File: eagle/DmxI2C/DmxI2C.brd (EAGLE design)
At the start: 55 x 69.5 mm, 30 parts, among them IC2 MAX485, IC3 MEGA48/88/168-AU, Q1 20MHz

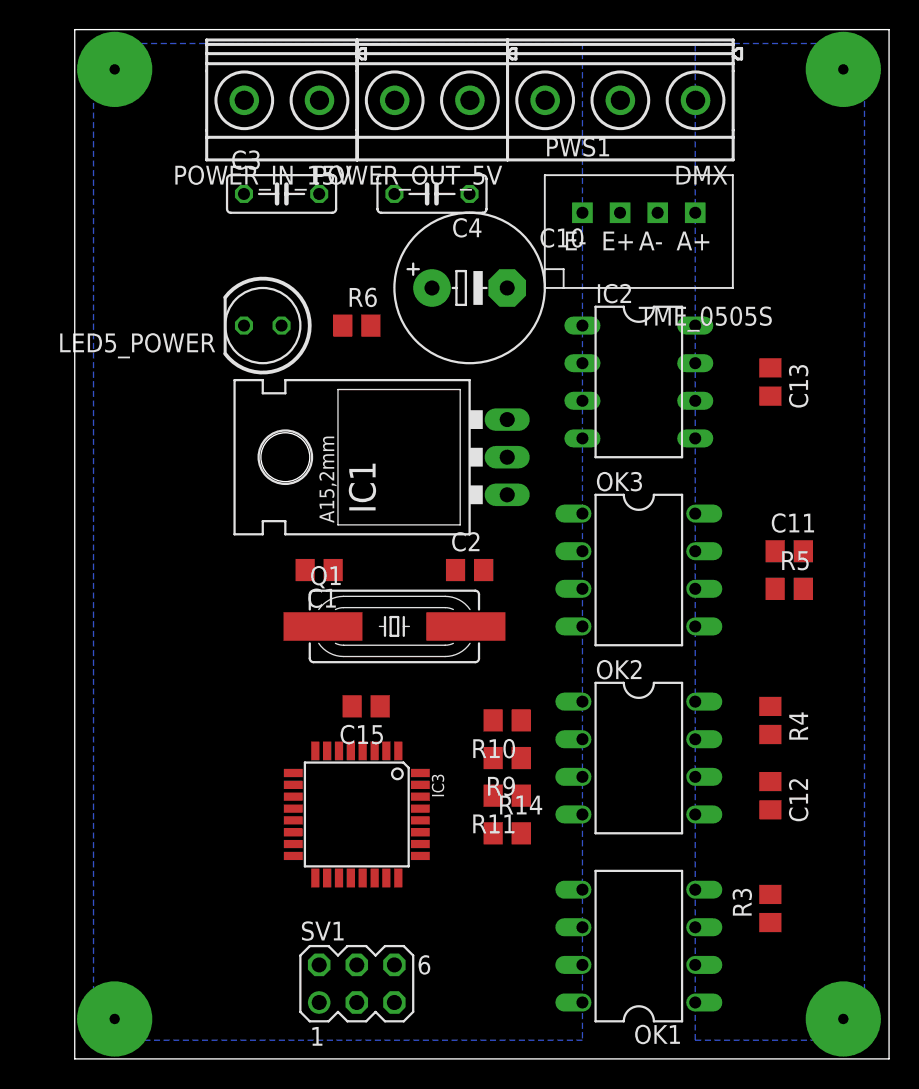
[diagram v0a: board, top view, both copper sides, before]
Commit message: .
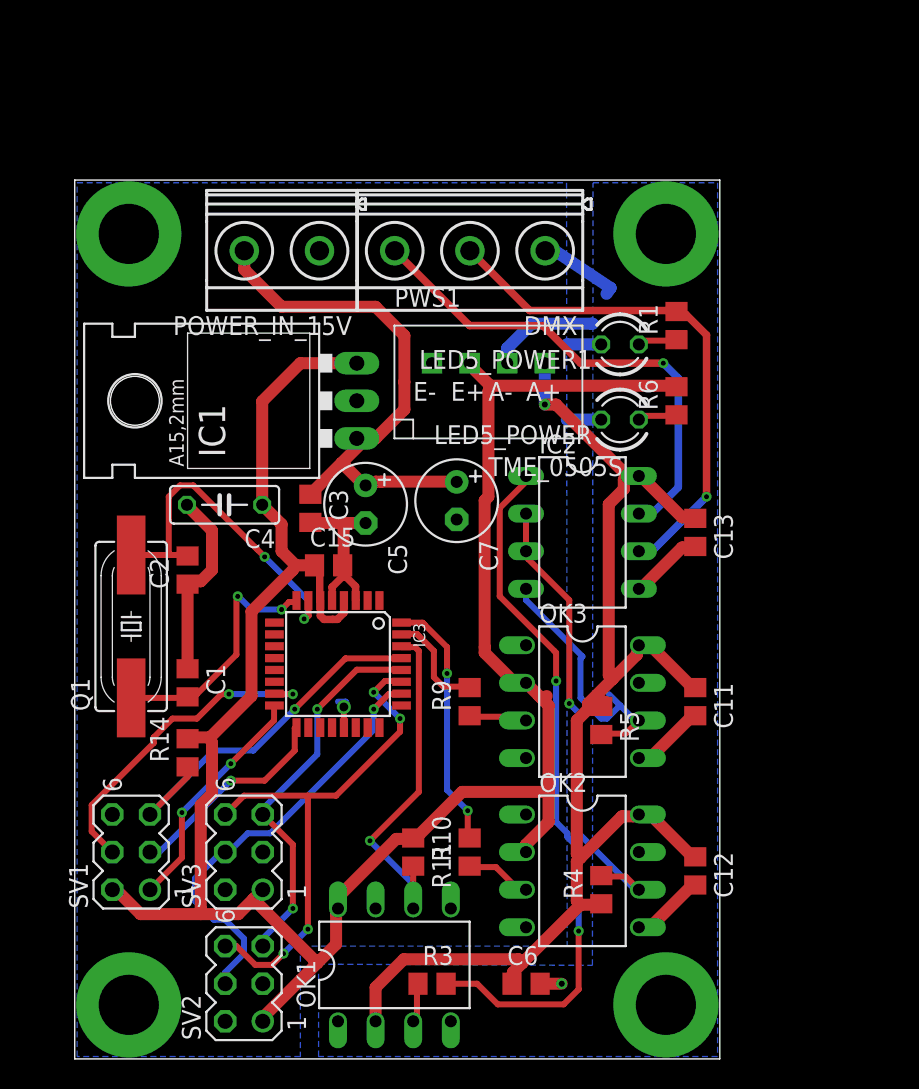
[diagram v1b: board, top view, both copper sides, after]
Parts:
- removed C10: 470µF, rcl:E5-10,5
- removed POWER_OUT_5V: MKDSN1,5/2-5,08, con-phoenix-508:MKDSN1,5/2-5,08
- added C5, C7: 470µF, rcl:E2,5-6
- added C6: 100nF, rcl:C0805
- added LED5_POWER1: (no value), led:LED3MM
- added R1: 300, rcl:R0805
- added SV2, SV3: (no value), con-lstb:MA03-2
- C3: device rcl:C050-025X075 -> rcl:C0805
- LED5_POWER: device led:LED5MM -> led:LED3MM
- moved C4 25.2 mm to (10.1, 37.4)
- moved LED5_POWER 25.0 mm to (36.8, 43.2)
- moved R3 23.4 mm to (24.1, 5.08), turned to 0 degrees
- moved R14 22.3 mm to (7.62, 20.7), turned to 90 degrees
- moved R6 22.2 mm to (40.6, 44.5), turned to 90 degrees
- moved C3 21.3 mm to (15.9, 37.2), turned to 270 degrees
- moved C2 19.1 mm to (7.62, 33.0), turned to 90 degrees
- moved Q1 17.8 mm to (3.81, 29.2), turned to 90 degrees
- moved SV1 17.6 mm to (3.81, 14.0), turned to 90 degrees
- moved OK1 16.6 mm to (21.6, 6.35), turned to 0 degrees
- moved R4 16.2 mm to (35.6, 11.4), turned to 90 degrees
- moved R5 15.5 mm to (35.6, 22.9), turned to 270 degrees
- moved PWS1 14.4 mm to (27.9, 45.7)
- moved DMX 14.4 mm to (24.1, 54.6)
- moved C11 12.0 mm to (41.9, 24.1), turned to 270 degrees
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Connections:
- net N$10 renamed DMX-
- removed net N$11: DMX.2, IC2.6
- new net DMX+: DMX.2, IC2.6, R1.2
- new net N$10: LED5_POWER1.A, R1.1
- new net OUT_EN: IC3.26, SV2.4, SV3.4
- new net SCL: IC3.28, SV2.5, SV3.5
- new net SDA: IC3.27, SV2.6, SV3.6
- net +15V: now also C5.+, C7.+; no longer C10.+
- net +5V: now also SV2.1, SV3.1; no longer POWER_OUT_5V.1
- net +5V/2: now also C6.1
- net GND: now also C5.-, C7.-, LED5_POWER1.K, SV2.2, SV3.2; no longer C10.-, POWER_OUT_5V.2
- net GND2: now also C6.2
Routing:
- net +5V: track 0.00 -> 149.7 mm
- net +5V/2: track 0.00 -> 89.2 mm, vias 0 -> 1
- net N$2: track 0.00 -> 47.6 mm, vias 0 -> 2
- net +15V: track 0.00 -> 37.0 mm
- net SDA: track 0.00 -> 35.9 mm, vias 0 -> 4
- net DMX+: track 0.00 -> 35.4 mm, vias 0 -> 1
- net DMX-: track 0.00 -> 33.5 mm, vias 0 -> 1
- net N$3: track 0.00 -> 31.7 mm, vias 0 -> 1
- net GND: track 0.00 -> 31.2 mm, vias 0 -> 1
- net GND2: track 0.00 -> 29.7 mm, vias 0 -> 1
- net OUT_EN: track 0.00 -> 29.5 mm, vias 0 -> 1
- net SCL: track 0.00 -> 26.0 mm, vias 0 -> 2
- net RESET: track 0.00 -> 25.6 mm, vias 0 -> 1
- net N$7: track 0.00 -> 24.1 mm, vias 0 -> 1
- net N$9: track 0.00 -> 23.5 mm, vias 0 -> 2
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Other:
- board size 55 x 69.5 mm -> 43.6 x 59.4 mm
